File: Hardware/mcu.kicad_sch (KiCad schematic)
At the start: 20 parts, among them J1 I2C Debug, J2 Screen, J3 SPI Debug, SW1 TRIGGER, SW2 RESET, U6 ESP32-DevKitC

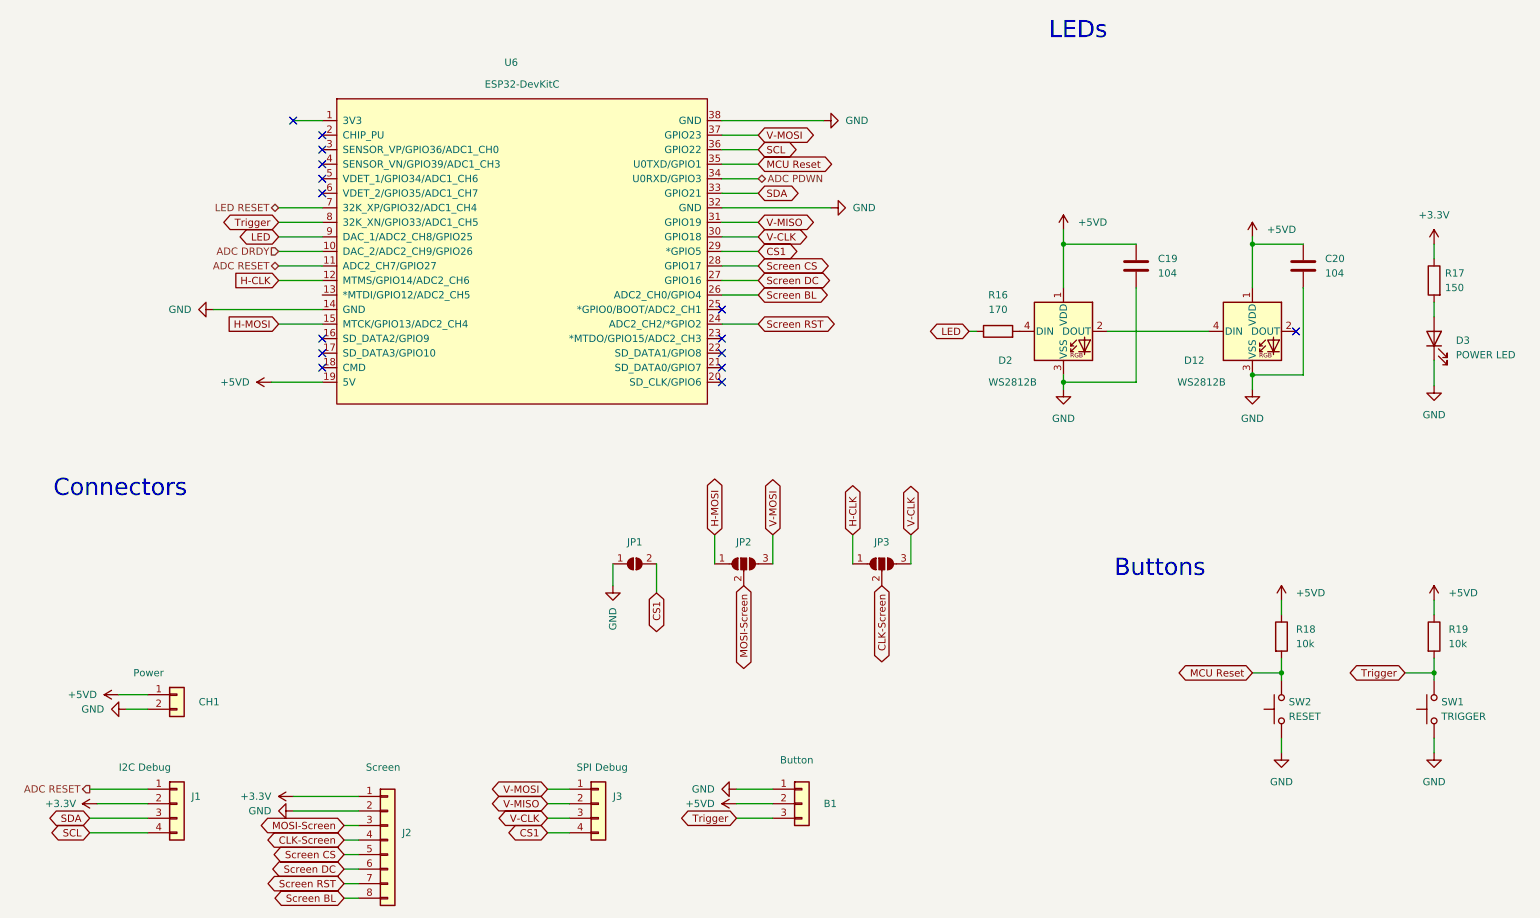
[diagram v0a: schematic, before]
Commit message: Version 0.1
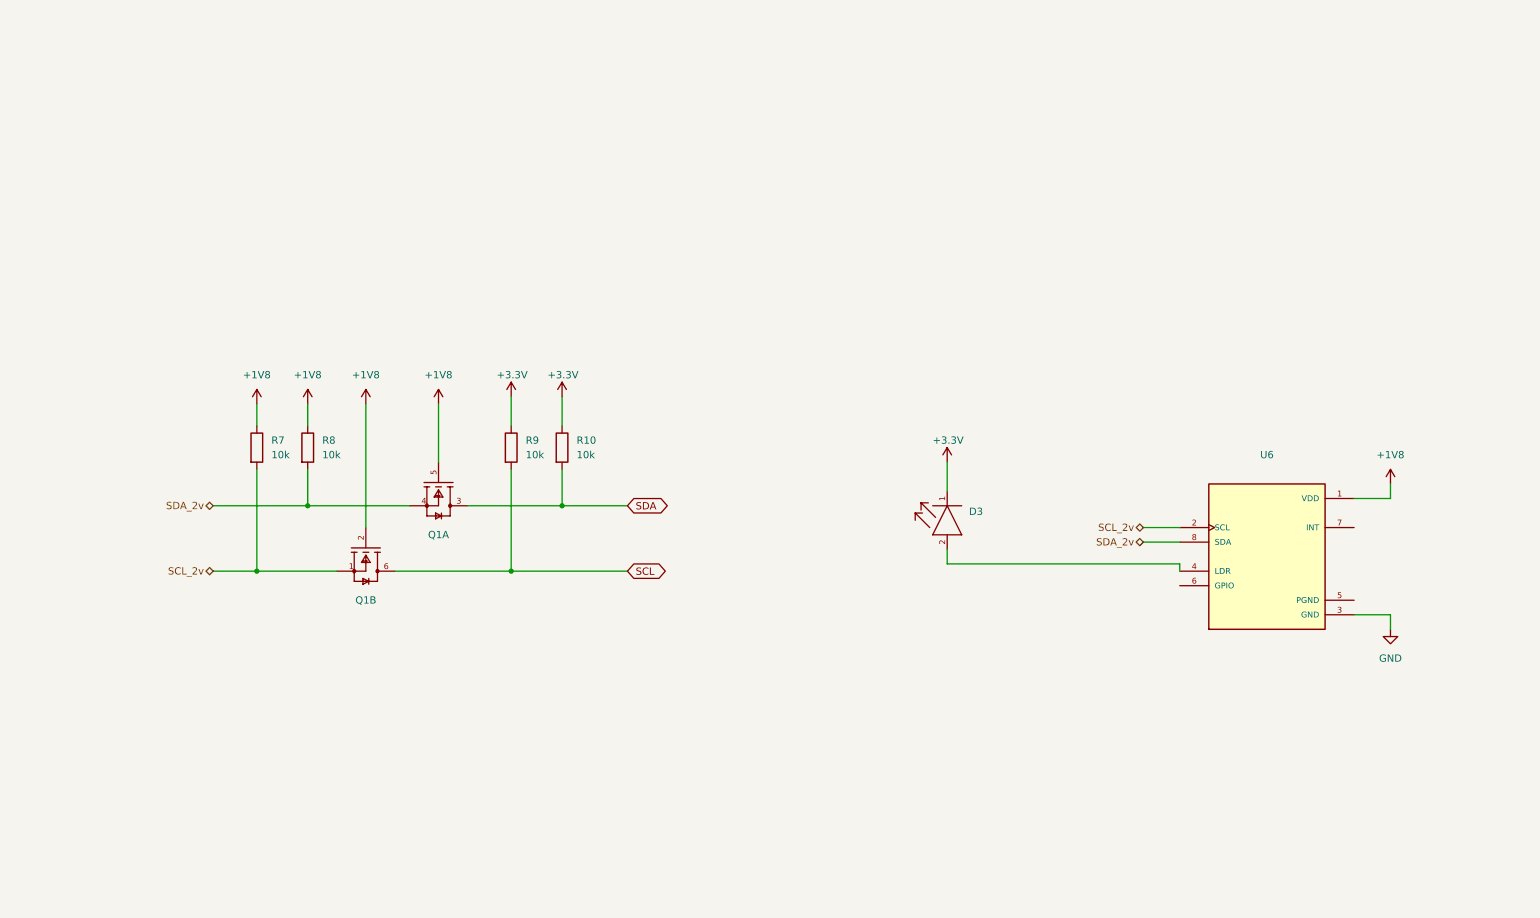
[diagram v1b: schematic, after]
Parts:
- removed B1: Button, Connector_JST:JST_SH_BM04B-SRSS-TB_1x04-1MP_P1.00mm_Vertical, symbol Connector_Generic:Conn_01x03
- removed C19, C20: 104, Capacitor_SMD:C_0805_2012Metric_Pad1.18x1.45mm_HandSolder, symbol Device:C
- removed CH1: Power, Connector_JST:JST_XH_B2B-XH-A_1x02_P2.50mm_Vertical, symbol Connector_Generic:Conn_01x02
- removed D12, D2: WS2812B, LED_SMD:LED_WS2812B_PLCC4_5.0x5.0mm_P3.2mm, symbol LED:WS2812B
- removed D3: POWER LED, LED_SMD:LED_0805_2012Metric_Pad1.15x1.40mm_HandSolder, symbol Device:LED
- removed J1: I2C Debug, Connector_JST:JST_XH_B4B-XH-A_1x04_P2.50mm_Vertical, symbol Connector_Generic:Conn_01x04
- removed J2: Screen, Connector_JST:JST_XH_S8B-XH-A_1x08_P2.50mm_Horizontal, symbol Connector_Generic:Conn_01x08
- removed J3: SPI Debug, Connector_JST:JST_XH_B4B-XH-A_1x04_P2.50mm_Vertical, symbol Connector_Generic:Conn_01x04
- removed JP1: SolderJumper_2_Open, Jumper:SolderJumper-2_P1.3mm_Open_TrianglePad1.0x1.5mm, symbol Jumper:SolderJumper_2_Open
- removed JP2, JP3: SolderJumper_3_Open, Jumper:SolderJumper-3_P2.0mm_Open_TrianglePad1.0x1.5mm_NumberLabels, symbol Jumper:SolderJumper_3_Open
- removed R16: 170, Resistor_SMD:R_0805_2012Metric_Pad1.20x1.40mm_HandSolder, symbol Device:R
- removed R17: 150, Resistor_SMD:R_0805_2012Metric_Pad1.20x1.40mm_HandSolder, symbol Device:R
- removed R18, R19: 10k, Resistor_SMD:R_0805_2012Metric_Pad1.20x1.40mm_HandSolder, symbol Device:R
- removed SW1: TRIGGER, Button_Switch_THT:SW_PUSH_6mm, symbol Switch:SW_Push
- removed SW2: RESET, Button_Switch_THT:SW_PUSH_6mm, symbol Switch:SW_Push
- removed U6: ESP32-DevKitC, ESP32:ESP32-DevKitC, symbol Espressif:ESP32-DevKitC
- added D3: (no value), symbol Everlight-EAHC2835WD6:EAHC2835WD6
- added Q1: (no value), symbol Diodes_Inc._-_BSS138DW-7-F:BSS138DW-7-F
- added R10, R7, R8, R9: 10k, symbol Device:R
- added U6: (no value), symbol AS7341-DLGT:AS7341-DLGT
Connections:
- net +3V3: now also D3.1 (CATHODE), R10.1, R9.1
- net GND: now also U6.3 (GND)
- net SCL: now also Q1.6 (D2), R9.2
- net SDA: now also Q1.3 (D1), R10.2
- new net: D3.2 (ANODE), U6.4 (LDR)
- new net +1V8: Q1.2 (G2), Q1.5 (G1), R7.1, R8.1, U6.1 (VDD)
- new net SCL_2v: Q1.1 (S2), R7.2, U6.2 (SCL)
- new net SDA_2v: Q1.4 (S1), R8.2, U6.8 (SDA)
- no-connect marks 15 -> 0
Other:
- note removed: "Buttons"
- note removed: "Connectors"
- note removed: "LEDs"
